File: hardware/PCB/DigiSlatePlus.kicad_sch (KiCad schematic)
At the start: 40 parts, among them J1 Serial, J10 IO7, J2 USB_B, J6 Mains, J7 Timecode IN, J8 Timecode OUT, J9 MISO, Q4 2N2222, SW1 RotaryEncoder-SW, SW2 1, SW3 1, SW4 1, SW5 1, SW6 BOOT, U1 ESP32-S3-WROOM-1, U2 DS3231M

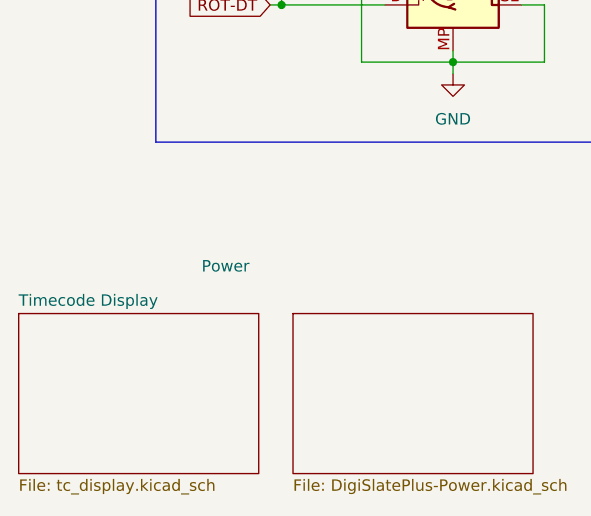
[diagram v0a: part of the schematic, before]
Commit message: final 1.0 board version
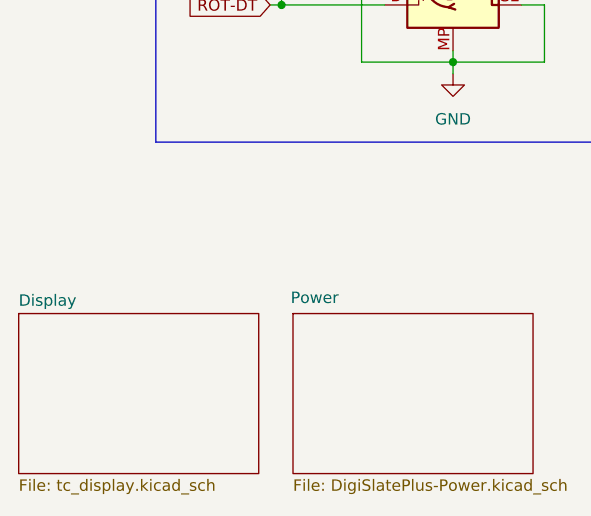
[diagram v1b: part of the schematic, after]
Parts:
- SW2, SW3, SW4, SW5: footprint Button_Switch_THT:SW_PUSH-12mm -> Button_Switch_THT:SW_Tactile_Straight_KSA0Axx1LFTR
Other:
- sheet Timecode Display renamed Display
- title: DigiSlatePlus -> DigiSlate+
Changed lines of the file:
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@@
 	(paper "A4")
 	(title_block
-		(title "DigiSlatePlus")
+		(title "DigiSlate+")
+		(date "2024-09-05")
 		(rev "1.0")
 	)
@@
 			)
 		)
-		(property "Footprint" "Button_Switch_THT:SW_PUSH-12mm"
+		(property "Footprint" "Button_Switch_THT:SW_Tactile_Straight_KSA0Axx1LFTR"
 			(at 114.3 152.4 0)
 			(effects
@@
 			)
 		)
-		(property "Footprint" "Button_Switch_THT:SW_PUSH-12mm"
+		(property "Footprint" "Button_Switch_THT:SW_Tactile_Straight_KSA0Axx1LFTR"
 			(at 124.46 152.4 0)
 			(effects
@@
 			)
 		)
-		(property "Footprint" "Button_Switch_THT:SW_PUSH-12mm"
+		(property "Footprint" "Button_Switch_THT:SW_Tactile_Straight_KSA0Axx1LFTR"
 			(at 104.14 152.4 0)
 			(effects
@@
 			)
 		)
-		(property "Footprint" "Button_Switch_THT:SW_PUSH-12mm"
+		(property "Footprint" "Button_Switch_THT:SW_Tactile_Straight_KSA0Axx1LFTR"
 			(at 134.62 152.4 0)
 			(effects
@@
 			(color 0 0 0 0.0000)
 		)
-		(property "Sheetname" "Timecode Display"
+		(property "Sheetname" "Display"
 			(at 17.78 173.2784 0)
 			(effects
@@
 		)
 		(property "Sheetname" "Power"
-			(at 38.1 169.4684 0)
+			(at 48.006 172.974 0)
 			(effects
 				(font
